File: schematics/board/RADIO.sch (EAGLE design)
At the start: 50 parts, among them J1 IPX-RADIO, J2 IPX-ANT

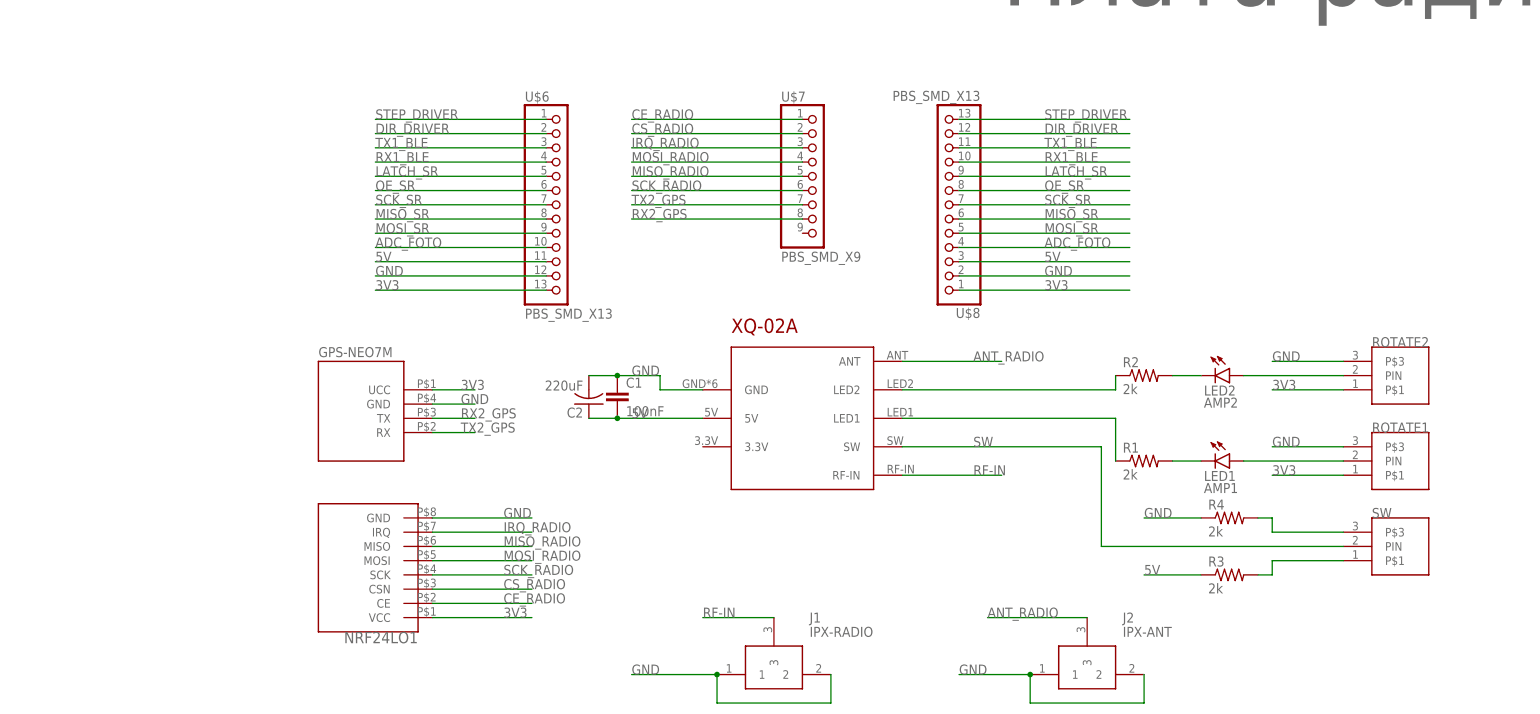
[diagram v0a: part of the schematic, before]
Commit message: Платки там
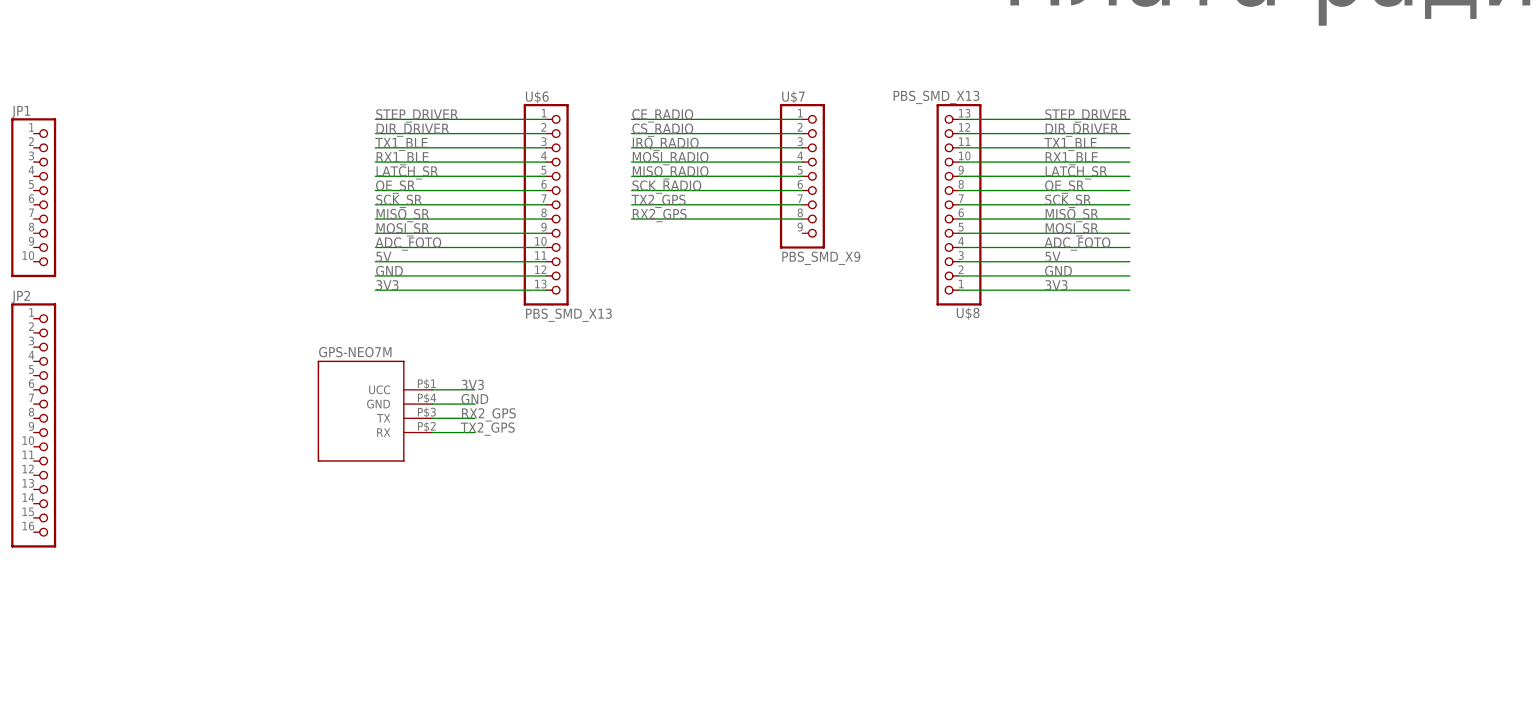
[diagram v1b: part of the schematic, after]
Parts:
- removed C1: 100nF, rcl:C-EUC0603
- removed C2: 220uF, UNKNOWN-2024:ECAPECAP220
- removed J1: IPX-RADIO, UNKNOWN-2024:U.FL-R-SMT-1_10_
- removed J2: IPX-ANT, UNKNOWN-2024:U.FL-R-SMT-1_10_
- removed LED1: AMP1, led:LEDCHIPLED_0603
- removed LED2: AMP2, led:LEDCHIPLED_0603
- removed NRF24LO1: NRF24L01_ML01SP4, UNKNOWN-2024:NRF24L01_ML01SP4
- removed R1, R2, R3, R4: 2k, rcl:R-US_R0603
- removed ROTATE1, ROTATE2, SW: CONNECT_3, UNKNOWN-2024:CONNECT_3
- removed XQ-02A: XQ-02A, UNKNOWN-2024:XQ-02A
- added JP1: (no value), pinhead:PINHD-1X10
- added JP2: (no value), pinhead:PINHD-1X16
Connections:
- removed net ANT_RADIO: J2.3, XQ-02A.ANT
- removed net N$1: LED1.C, R1.2
- removed net N$2: LED2.C, R2.2
- removed net N$3: LED1.A, ROTATE1.PIN
- removed net N$4: LED2.A, ROTATE2.PIN
- removed net N$5: R2.1, XQ-02A.LED2
- removed net N$6: R1.1, XQ-02A.LED1
- removed net N$7: R3.2, SW.P$1
- removed net N$8: R4.2, SW.P$3
- removed net RF-IN: J1.3, XQ-02A.RF-IN
- removed net SW: SW.PIN, XQ-02A.SW
- net 3V3: no longer NRF24LO1.VCC, ROTATE1.P$1, ROTATE2.P$1
- net 5V: no longer C1.2, C2.1, R3.1, XQ-02A.5V
- net CE_RADIO: no longer NRF24LO1.CE
- net CS_RADIO: no longer NRF24LO1.CSN
- net GND: no longer C1.1, C2.2, J1.1, J1.2, J2.1, J2.2, NRF24LO1.GND, R4.1, ROTATE1.P$3, ROTATE2.P$3, XQ-02A.GND
- net IRQ_RADIO: no longer NRF24LO1.IRQ
- net MISO_RADIO: no longer NRF24LO1.MISO
- net MOSI_RADIO: no longer NRF24LO1.MOSI
- net SCK_RADIO: no longer NRF24LO1.SCK

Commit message: ПЛАТЫ, АААААААААААААААААААААААААААА
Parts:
- added JP3: (no value), pinhead:PINHD-1X18
- added R1: 10k, rcl:R-US_R0603
- added R2: 100R, rcl:R-US_R0603
- added S1: (no value), UNKNOWN-2024:UNICS-SWITCHSS_12D11
- added SI2302CDS: SI2302CDS, CanCubeSat:SI2302CDS
- added U$10: LIS3MDL, UNKNOWN-2024:LIS3MDL
- added U$18: MOLEX-2-1.25, UNKNOWN-2024:MOLEX-2-1.25
- added U$4: E220-400T22S, UNKNOWN-2024:E220-400T22S
- added U$9: LSM6DS3_WITHOUT, UNKNOWN-2024:LSM6DS3_WITHOUT
- added X2: AKKUM, UNKNOWN-2024:JST-2-2.5
- JP2: device pinhead:PINHD-1X16 -> pinhead:PINHD-1X8
- U$6: value PBS_SMD_X13 -> MOLEX-2-1.25; device UNKNOWN-2024:PBS_SMD_X13 -> UNKNOWN-2024:MOLEX-2-1.25
- U$7: value PBS_SMD_X9 -> MOLEX-2-1.25; device UNKNOWN-2024:PBS_SMD_X9 -> UNKNOWN-2024:MOLEX-2-1.25
- U$8: value PBS_SMD_X13 -> JST-6-2.5; device UNKNOWN-2024:PBS_SMD_X13 -> UNKNOWN-2024:JST-6-2.5
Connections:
- removed net ADC_FOTO: U$6.10, U$8.4
- removed net CE_RADIO: U$7.1
- removed net CS_RADIO: U$7.2
- removed net DIR_DRIVER: U$6.2, U$8.12
- removed net IRQ_RADIO: U$7.3
- removed net LATCH_SR: U$6.5, U$8.9
- removed net MISO_RADIO: U$7.5
- removed net MOSI_RADIO: U$7.4
- removed net OE_SR: U$6.6, U$8.8
- removed net RX1_BLE: U$6.4, U$8.10
- removed net RX2_GPS: GPS-NEO7M.TX, U$7.8
- removed net SCK_RADIO: U$7.6
- removed net STEP_DRIVER: U$6.1, U$8.13
- removed net TX1_BLE: U$6.3, U$8.11
- removed net TX2_GPS: GPS-NEO7M.RX, U$7.7
- new net 3V7: JP1.10
- new net AUX_RADIO: JP3.10, U$4.AUX
- new net BUS+_OUT: S1.S, X2.1
- new net C0: JP2.1, JP3.1
- new net CS_LIS: JP1.8, U$10.CS
- new net CS_LSM: JP1.9, U$9.CS
- new net GERMO: JP3.18, R2.1
- new net LATCH: JP1.5, U$8.1
- new net M0_RADIO: JP3.12, U$4.M0
- new net M1_RADIO: JP3.11, U$4.M1
- new net MICS: JP2.4, JP3.4
- new net MISO_SENS: JP1.2
- new net MOSI: U$8.3
- new net MOSI_SENS: JP1.1
- new net N$2: R1.1, R2.2, SI2302CDS.G
- new net N$5: SI2302CDS.D, U$18.1, U$6.1, U$7.1
- new net NH3: JP2.3, JP3.3
- new net NO2: JP2.2, JP3.2
- new net OE: JP1.4, U$8.P$1
- new net RX_GPS: GPS-NEO7M.TX, JP3.14
- new net RX_LIDAR: JP3.15
- new net RX_RADIO: JP1.6, U$4.TXD
- new net SCK: U$8.2
- new net SCK_SENS: JP1.3
- new net SCL: JP2.8, JP3.9
- new net SDA: JP2.7, JP3.8
- new net SHIFT2: U$8.P$2
- new net SHIFT_2: JP3.17
- new net TX_GPS: GPS-NEO7M.RX, JP3.13
- new net TX_LIDAR: JP3.16
- new net TX_RADIO: JP1.7, U$4.RXD
- net 3V3: now also JP3.6, U$10.UCC, U$4.VCC, U$8.4, U$9.3V3; no longer U$6.13, U$8.1
- net 5V: now also JP2.6, JP3.7, U$18.2, U$6.2, U$7.2; no longer U$6.11, U$8.3
- net BUS+: now also S1.P
- net GND: now also JP2.5, JP3.5, R1.2, SI2302CDS.S, U$10.GND, U$4.GND, U$9.GND, X2.2; no longer U$6.12, U$8.2
- net MISO_SR: now also U$10.SDO, U$9.CAO; no longer U$6.8, U$8.6
- net MOSI_SR: now also U$10.SDA, U$9.SDA; no longer U$6.9, U$8.5
- net SCK_SR: now also U$10.SCL, U$9.SCL; no longer U$6.7, U$8.7
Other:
- moved on the sheet: 3V3, 5V, C10, C11, C12, C13, C14, C15, C16, C3, C4, C5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
